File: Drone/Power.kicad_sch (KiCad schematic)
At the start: 11 parts, among them J3 USB_C_Receptacle_USB2.0, P9 CONN_1, U6 NUF2221, U9 TPS79301

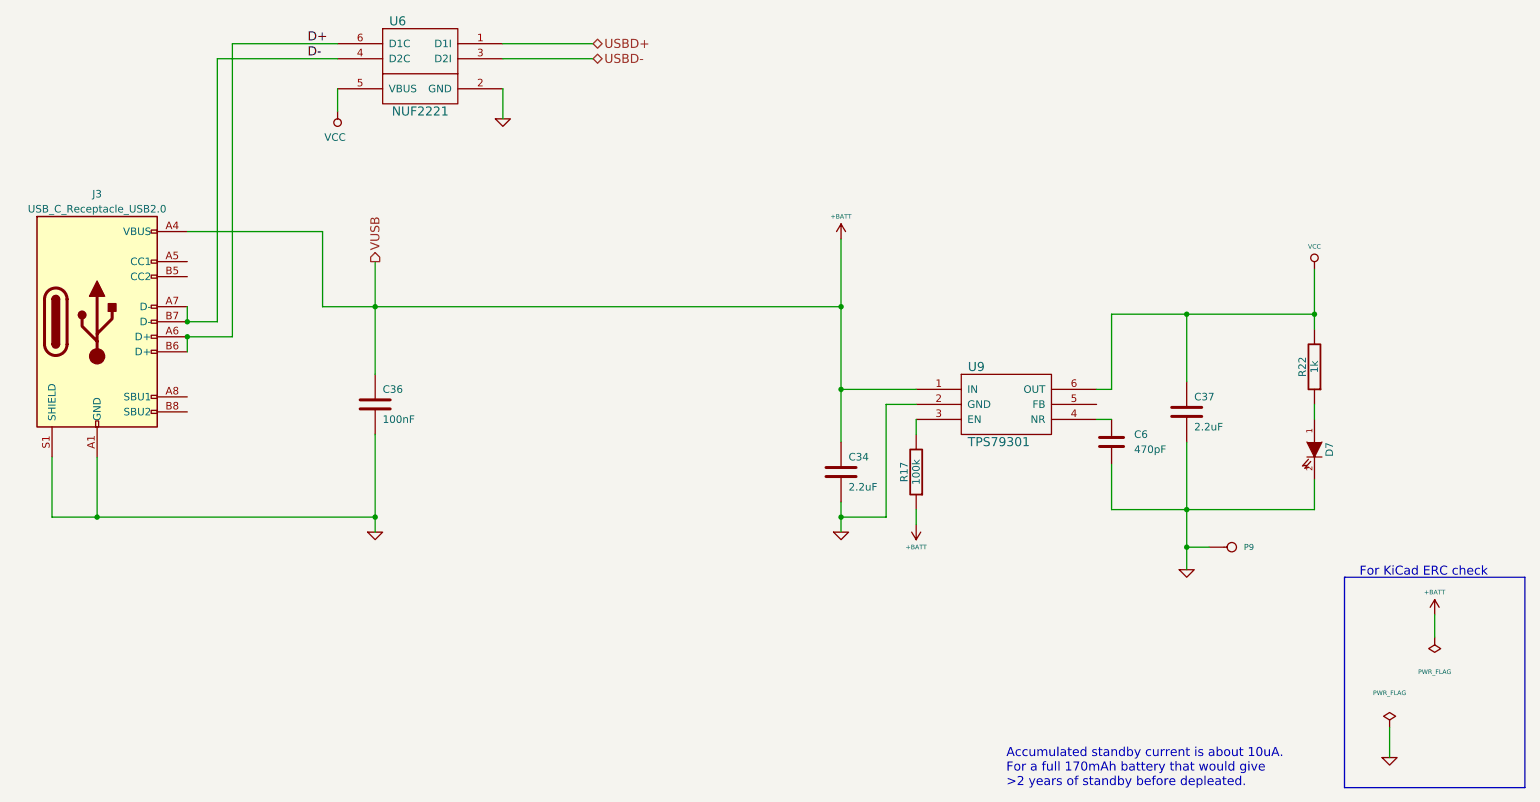
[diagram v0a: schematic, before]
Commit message: save
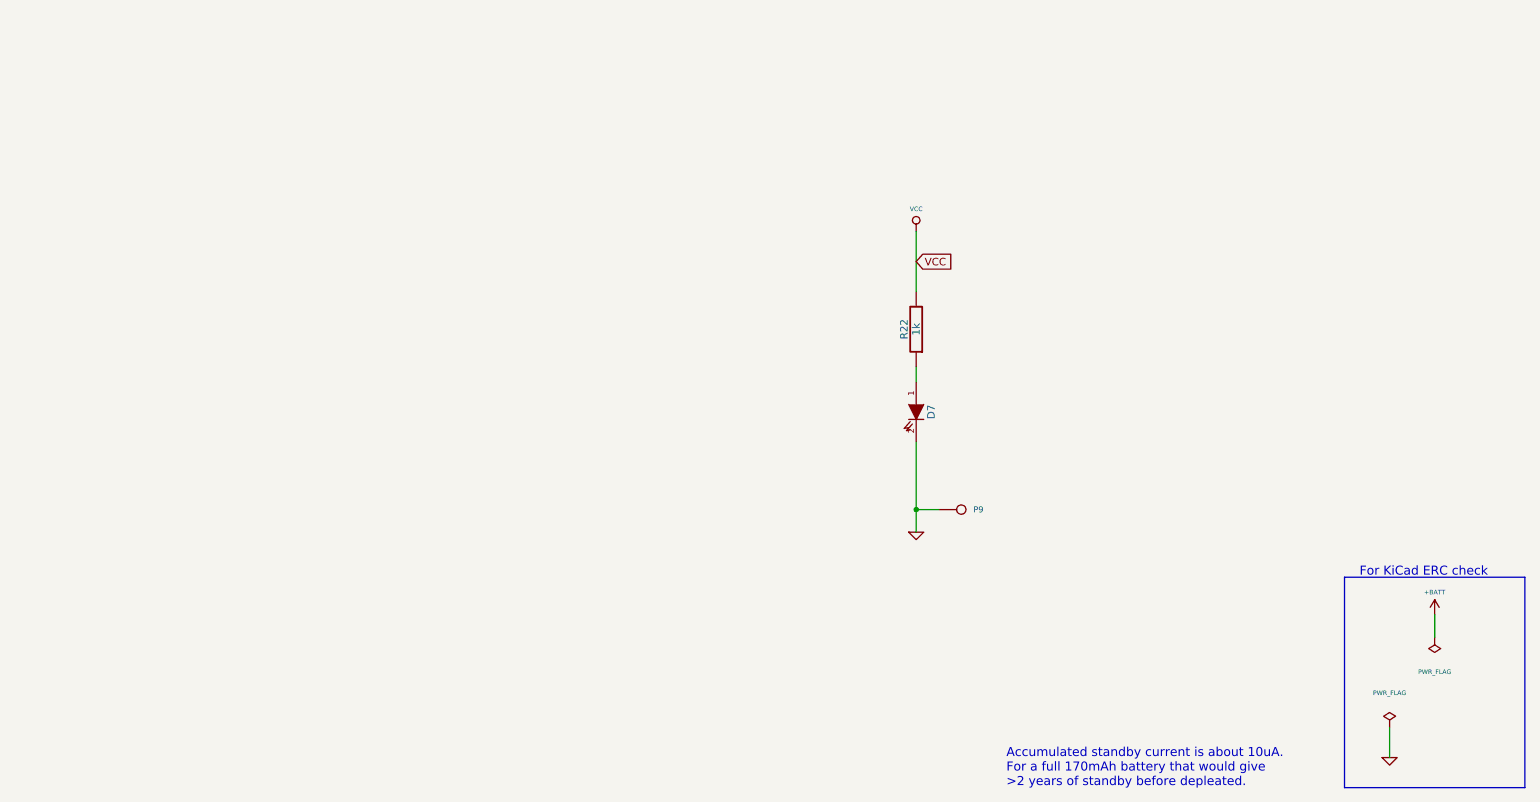
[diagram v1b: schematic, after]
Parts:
- removed C34, C37: 2.2uF, Capacitor_SMD:C_0603_1608Metric, symbol Crazyflie-contol-board-rescue:C-Crazyflie-contol-board-rescue
- removed C36: 100nF, Capacitor_SMD:C_0603_1608Metric, symbol Crazyflie-contol-board-rescue:C-Crazyflie-contol-board-rescue
- removed C6: 470pF, Capacitor_SMD:C_0603_1608Metric, symbol Device:C
- removed J3: USB_C_Receptacle_USB2.0, Connector_USB:USB_C_Receptacle_HRO_TYPE-C-31-M-12, symbol Connector:USB_C_Receptacle_USB2.0
- removed R17: 100k, Resistor_SMD:R_0603_1608Metric, symbol Crazyflie-contol-board-rescue:R-Crazyflie-contol-board-rescue
- removed U6: NUF2221, SOT363, symbol Crazyflie-contol-board-rescue:NUF2221-Crazyflie-contol-board-rescue
- removed U9: TPS79301, SOT23_6, symbol Crazyflie-contol-board-rescue:TPS79301-Crazyflie-contol-board-rescue
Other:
- moved on the sheet: D7, P9, R22
